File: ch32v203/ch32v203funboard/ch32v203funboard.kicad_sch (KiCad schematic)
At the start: 21 parts, among them J1 HDR, J3 PGM, J4 USB_C_Receptacle_USB2.0, J5 HDR, SW1 BOOT, U2 SRV05-4, U3 XC6206P332, Y2 8MHz

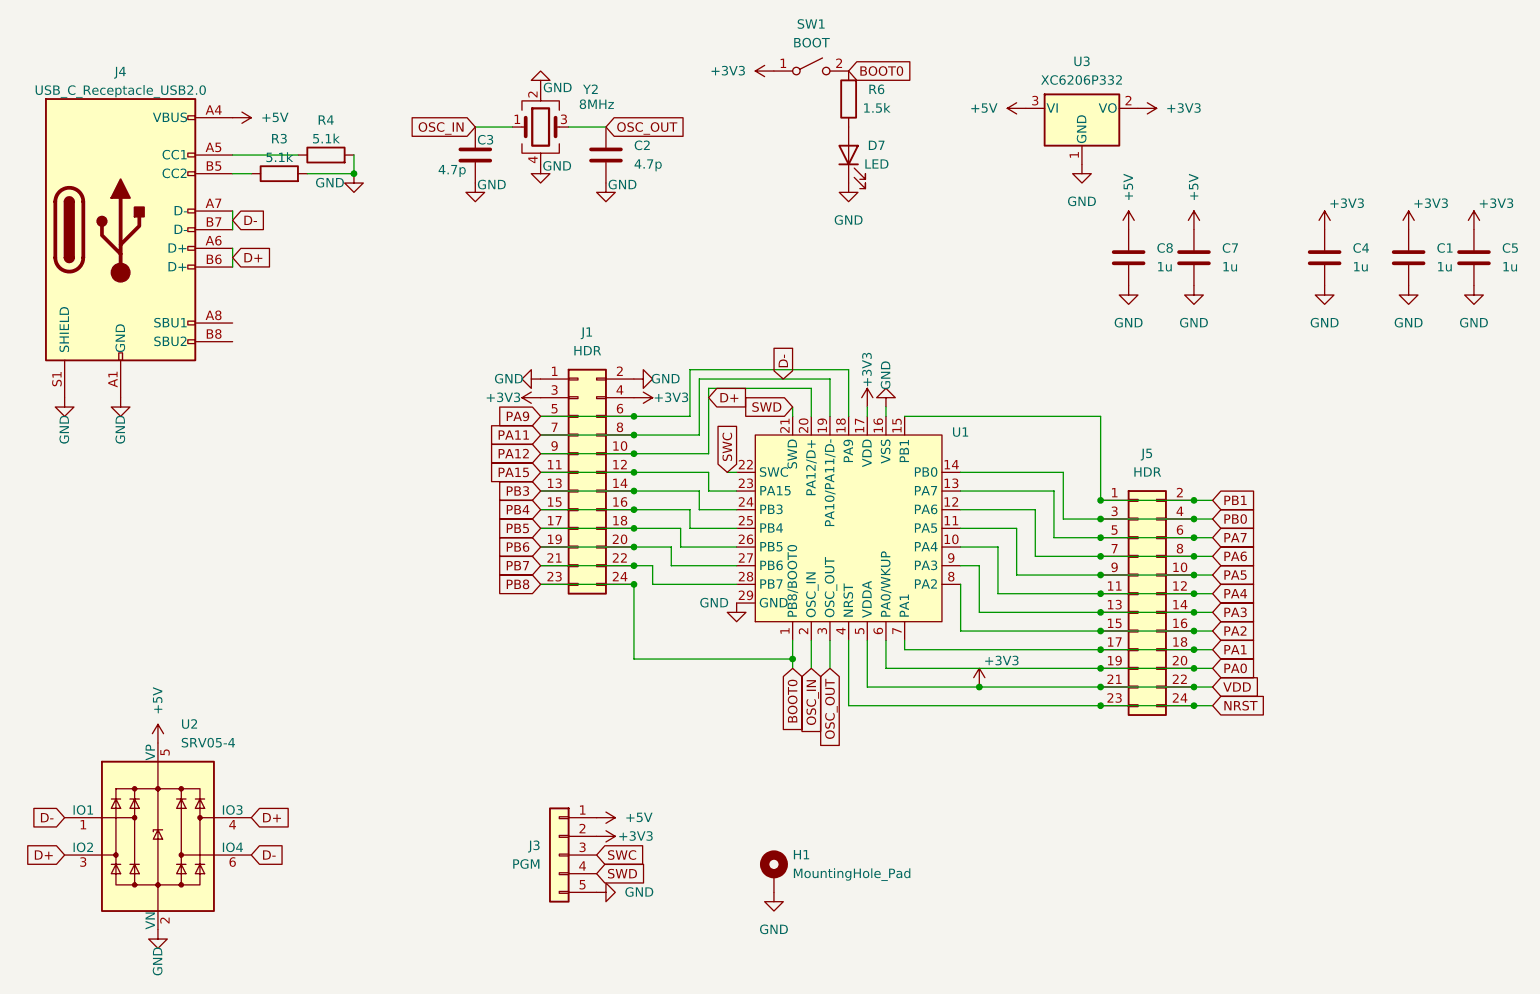
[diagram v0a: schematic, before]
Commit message: Bump board
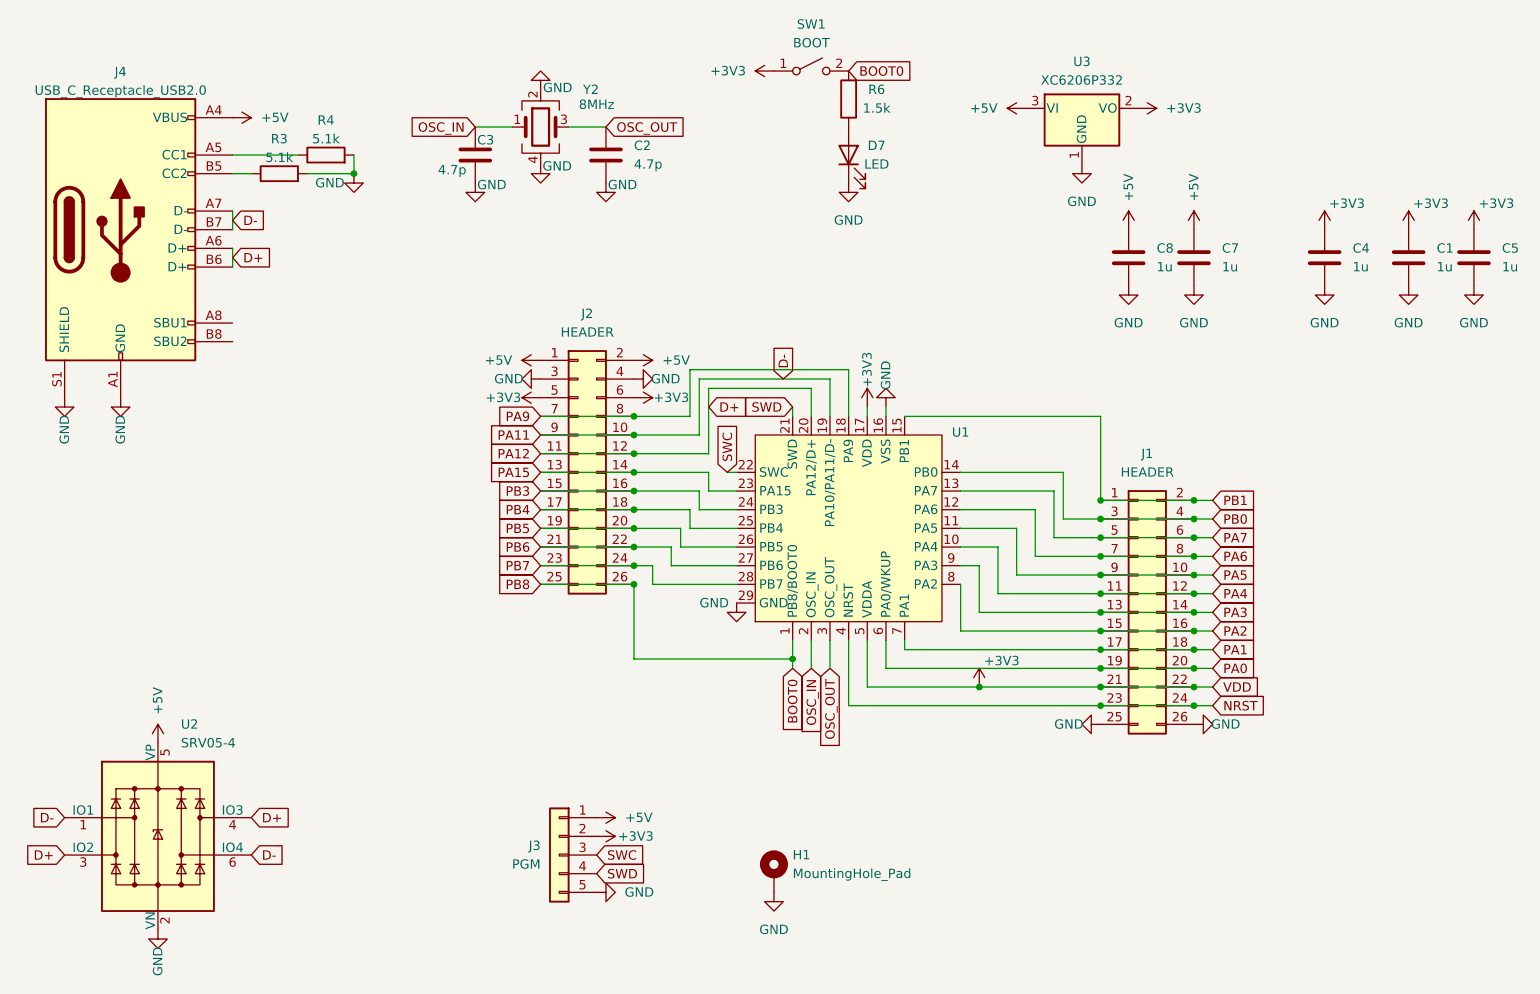
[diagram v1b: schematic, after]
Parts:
- removed J1, J5: HDR, Connector_PinHeader_2.54mm:PinHeader_2x12_P2.54mm_Vertical, symbol Connector_Generic:Conn_02x12_Odd_Even
- added J1, J2: HEADER, Connector_PinHeader_2.54mm:PinHeader_2x13_P2.54mm_Vertical, symbol Connector_Generic:Conn_02x13_Odd_Even
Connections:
- net +3V3: now also J1.21 (Pin_21), J1.22 (Pin_22), J2.5 (Pin_5), J2.6 (Pin_6)
- net +5V: now also J2.1 (Pin_1), J2.2 (Pin_2)
- net BOOT0: now also J2.25 (Pin_25), J2.26 (Pin_26)
- net D+: now also J2.11 (Pin_11), J2.12 (Pin_12)
- net D-: now also J2.10 (Pin_10), J2.9 (Pin_9)
- net GND: now also J1.25 (Pin_25), J1.26 (Pin_26), J2.3 (Pin_3), J2.4 (Pin_4)
- net NRST: now also J1.23 (Pin_23), J1.24 (Pin_24)
- net PA0: now also J1.19 (Pin_19), J1.20 (Pin_20)
- net PA1: now also J1.17 (Pin_17), J1.18 (Pin_18)
- net PA15: now also J2.13 (Pin_13), J2.14 (Pin_14)
- net PA2: now also J1.15 (Pin_15), J1.16 (Pin_16)
- net PA3: now also J1.13 (Pin_13), J1.14 (Pin_14)
- net PA4: now also J1.11 (Pin_11), J1.12 (Pin_12)
- net PA5: now also J1.10 (Pin_10), J1.9 (Pin_9)
- net PA6: now also J1.7 (Pin_7), J1.8 (Pin_8)
- net PA7: now also J1.5 (Pin_5), J1.6 (Pin_6)
- net PA9: now also J2.7 (Pin_7), J2.8 (Pin_8)
- net PB0: now also J1.3 (Pin_3), J1.4 (Pin_4)
- net PB1: now also J1.1 (Pin_1), J1.2 (Pin_2)
- net PB3: now also J2.15 (Pin_15), J2.16 (Pin_16)
- net PB4: now also J2.17 (Pin_17), J2.18 (Pin_18)
- net PB5: now also J2.19 (Pin_19), J2.20 (Pin_20)
- net PB6: now also J2.21 (Pin_21), J2.22 (Pin_22)
- net PB7: now also J2.23 (Pin_23), J2.24 (Pin_24)

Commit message: Bump designs
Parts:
- J3: LCSC (none) -> C492404
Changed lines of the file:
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@@
 			)
 		)
-		(property "LCSC" ""
+		(property "LCSC" "C492404"
 			(at 91.44 128.27 0)
 			(effects
